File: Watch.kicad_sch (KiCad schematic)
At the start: 46 parts, among them J1 USB_C_Receptacle_USB2.0_14P, Q1 2N3904, Q2 2N3904, Q3 2N3904, Q4 2N3904, SW1 SW_Push, SW3 SW_Push, SW4 SW_Push, U1 MCP73831-2-OT, U3 AP2112K-3.3, U7 ATSAMD21E18A-A, Y2 32768Hz

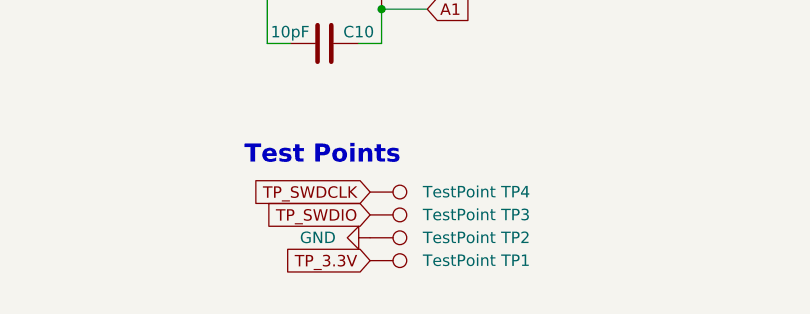
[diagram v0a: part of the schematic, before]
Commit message: Better test points
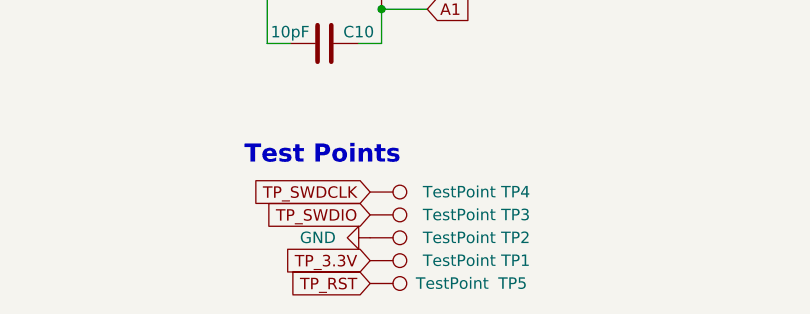
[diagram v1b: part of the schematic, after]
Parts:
- added TP5: TestPoint, symbol Connector:TestPoint
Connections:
- new net TP_RST: TP5.1
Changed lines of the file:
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@@
+		)
+	)
+	(global_label "TP_RST"
+		(shape input)
+		(at 171.45 240.03 180)
+		(fields_autoplaced yes)
+		(effects
+			(font
+				(size 1.27 1.27)
+			)
+			(justify right)
+		)
+		(property "Intersheetrefs" "${INTERSHEET_REFS}"
+			(at 161.8125 240.03 0)
+			(effects
+				(font
+					(size 1.27 1.27)
+				)
+				(justify right)
+				(hide yes)
+			)
 		)
 	)
@@
 					(unit 1)
 				)
+			)
+		)
+	)
+	(symbol
+		(lib_id "Connector:TestPoint")
+		(at 171.45 240.03 270)
+		(unit 1)
+		(exclude_from_sim no)
+		(in_bom yes)
+		(on_board yes)
+		(dnp no)
+		(property "Reference" "TP5"
+			(at 185.674 240.03 90)
+			(effects
+				(font
+					(size 1.27 1.27)
+				)
+				(justify left)
+			)
+		)
+		(property "Value" "TestPoint"
+			(at 176.53 240.03 90)
+			(effects
+				(font
+					(size 1.27 1.27)
+				)
+				(justify left)
+			)
+		)
+		(property "Footprint" ""
+			(at 171.45 245.11 0)
+			(effects
+				(font
+					(size 1.27 1.27)
+				)
+				(hide yes)
+			)
+		)
+		(property "Datasheet" "~"
+			(at 171.45 245.11 0)
+			(effects
+				(font
+					(size 1.27 1.27)
+				)
+				(hide yes)
+			)
+		)
+		(property "Description" "test point"
+			(at 171.45 240.03 0)
+			(effects
+				(font
+					(size 1.27 1.27)
+				)
+				(hide yes)
+			)
+		)
+		(pin "1"
+		)
+		(instances
+			(project ""
+				(path "/e5022d08-9dda-4e3a-b81c-bab3a6fb67af"
+					(reference "TP5")
+					(unit 1)
+				)
